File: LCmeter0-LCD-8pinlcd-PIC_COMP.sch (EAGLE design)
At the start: 34 parts, among them IC1 PIC16F876A-X/SP-COMP-B-A/V, J1 HD44780, J2 PIC-UART, J3 PIC-ICSPICSP, K2 DS2Y, Q1 20MHz, T1 BC547, X1 FREQ, X2 L/C

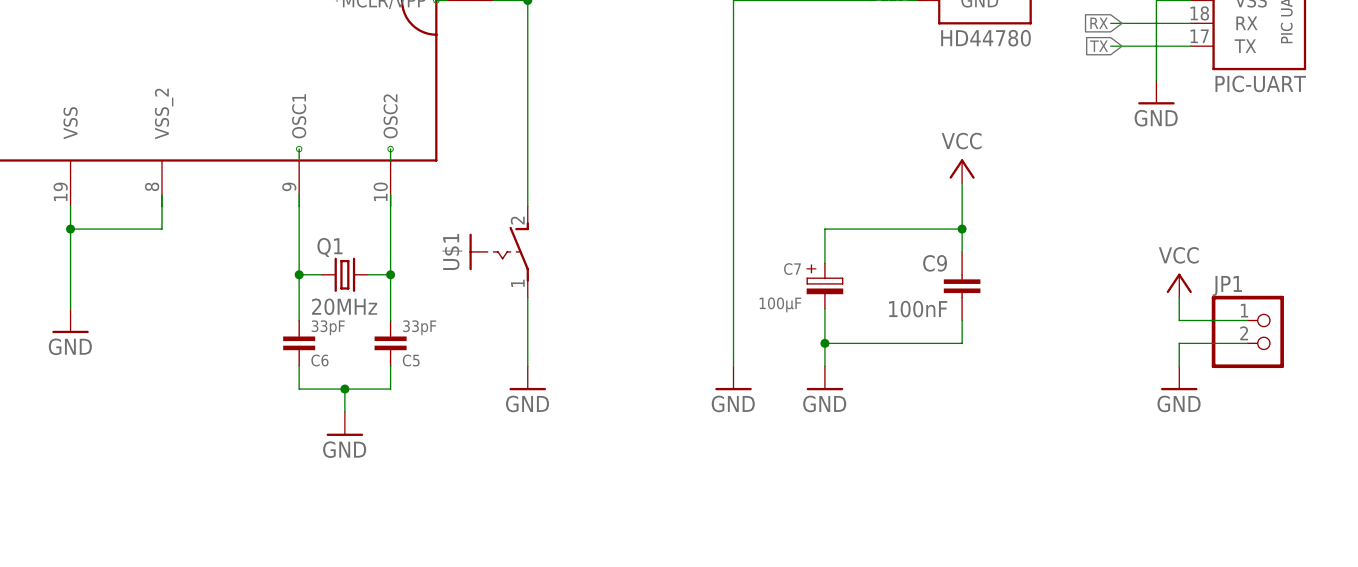
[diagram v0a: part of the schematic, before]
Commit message: ...
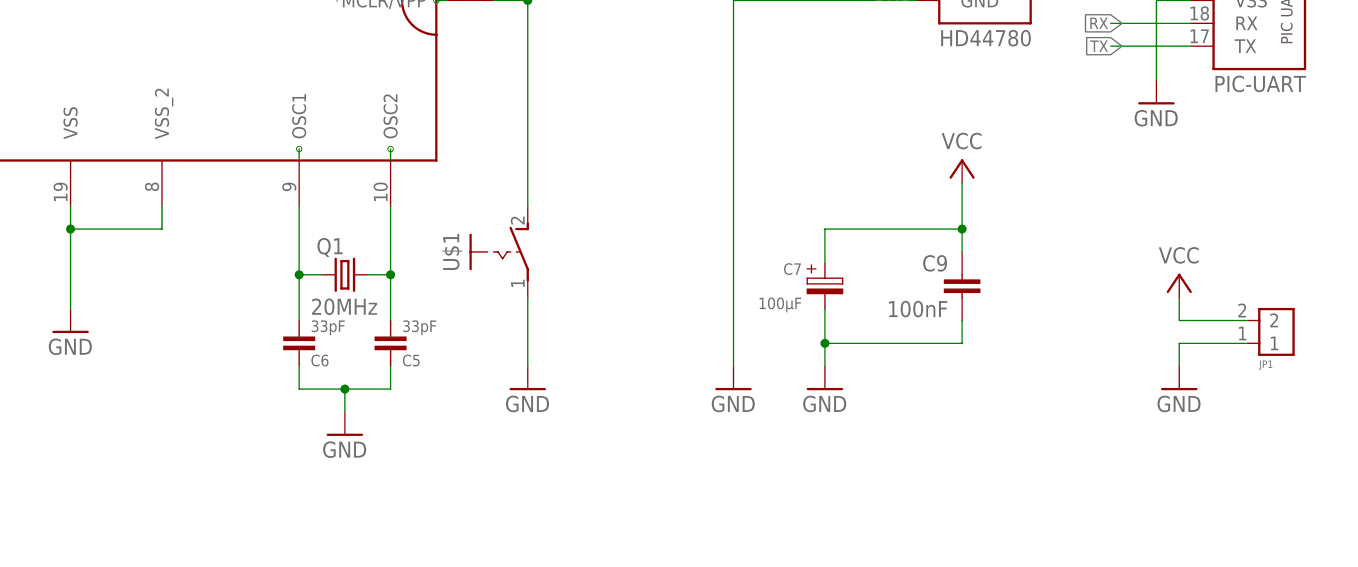
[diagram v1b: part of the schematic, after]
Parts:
- JP1: value (none) -> CONN-2P2P/V; device pinhead:PINHD-1X2 -> pinconn:CONN-2P2P/V
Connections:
- net GND: now also JP1.1; no longer JP1.2
- net VCC: now also JP1.2; no longer JP1.1

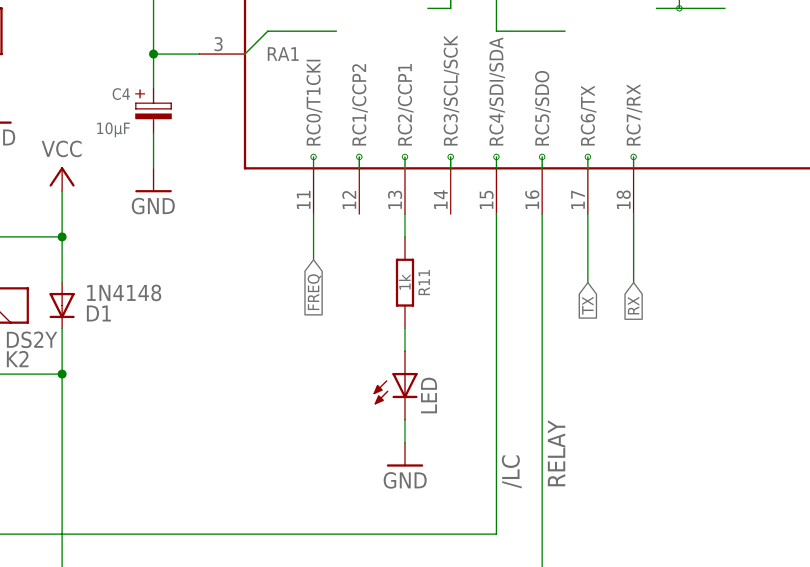
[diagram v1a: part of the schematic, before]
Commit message: ...
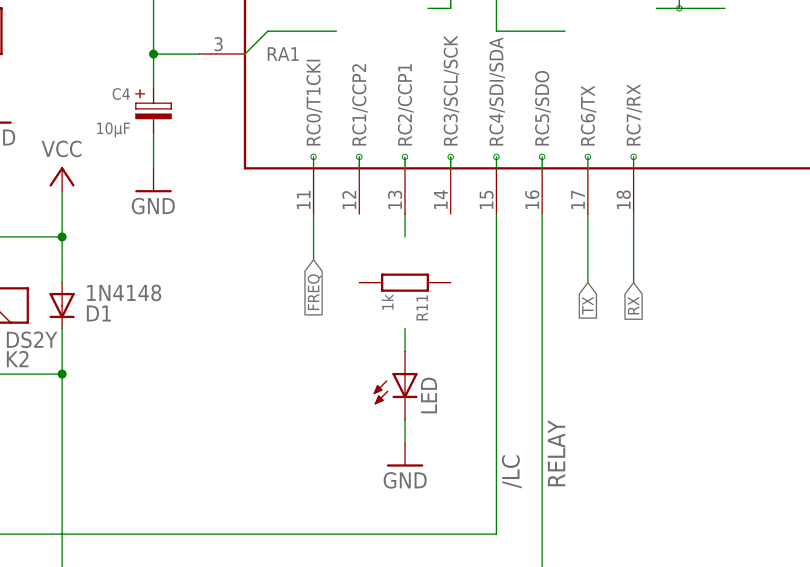
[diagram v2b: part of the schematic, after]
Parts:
- R11: device r:R-H0202/5 -> r:R0202/5
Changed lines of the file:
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@@
 <part name="R9" library="r" deviceset="R-H" device="0202/5" value="100"/>
 <part name="J1" library="pinconn" deviceset="HD44780-4BIT" device="-8PIN" value="HD44780"/>
-<part name="R11" library="r" deviceset="R-H" device="0202/5" value="1k"/>
+<part name="R11" library="r" deviceset="R" device="0202/5" value="1k"/>
 <part name="LED" library="led" deviceset="TLLG4400" device="" value=""/>
 <part name="GND10" library="supply1" deviceset="GND" device=""/>
